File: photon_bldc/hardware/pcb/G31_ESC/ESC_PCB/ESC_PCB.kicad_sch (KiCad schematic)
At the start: 21 parts, among them J1 PWM_Input, J2 Motor_Plus, J3 Motor_Minus, J4 Conn_01x08, U1 STM32G431K6Ux, U2 AMS1117-5.0, U3 AMS1117-3.3, U4 74AHC1G86, U5 74AHC1G86

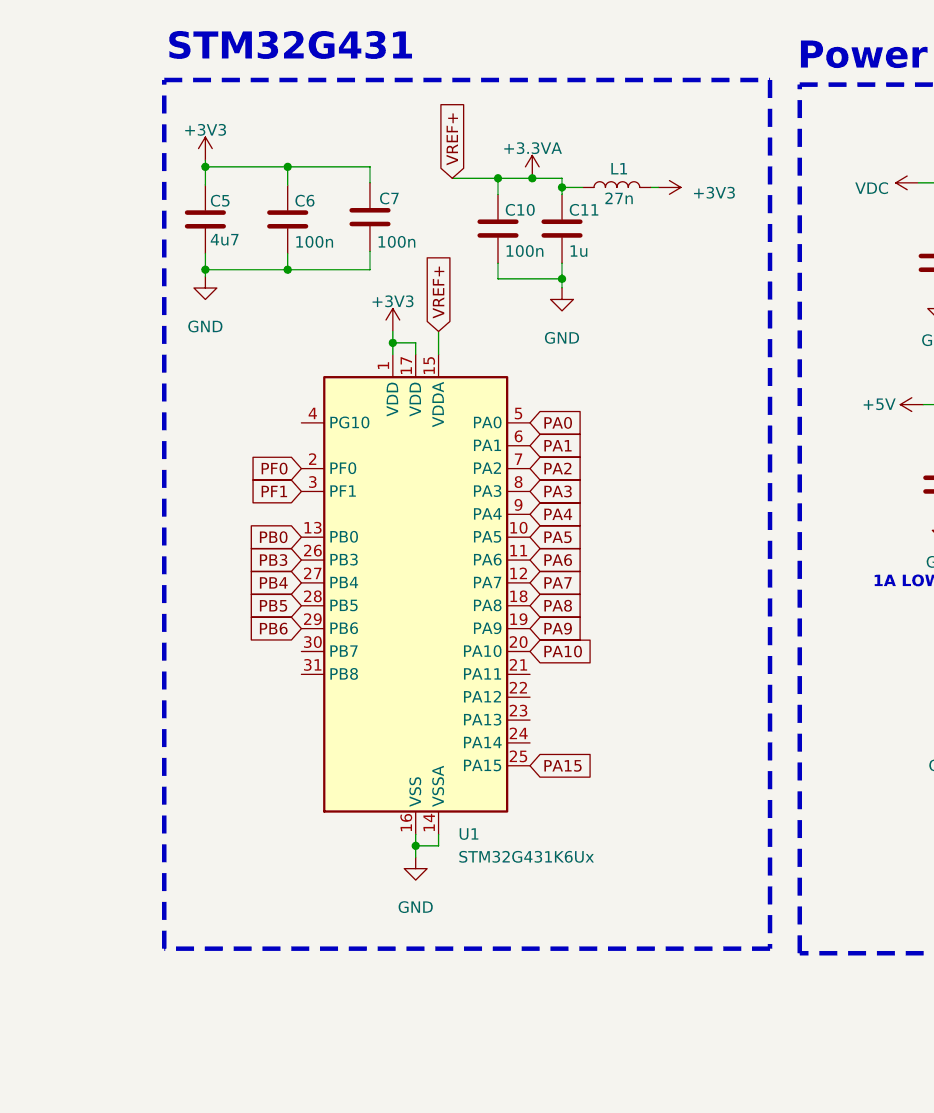
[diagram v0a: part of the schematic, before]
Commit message: g071
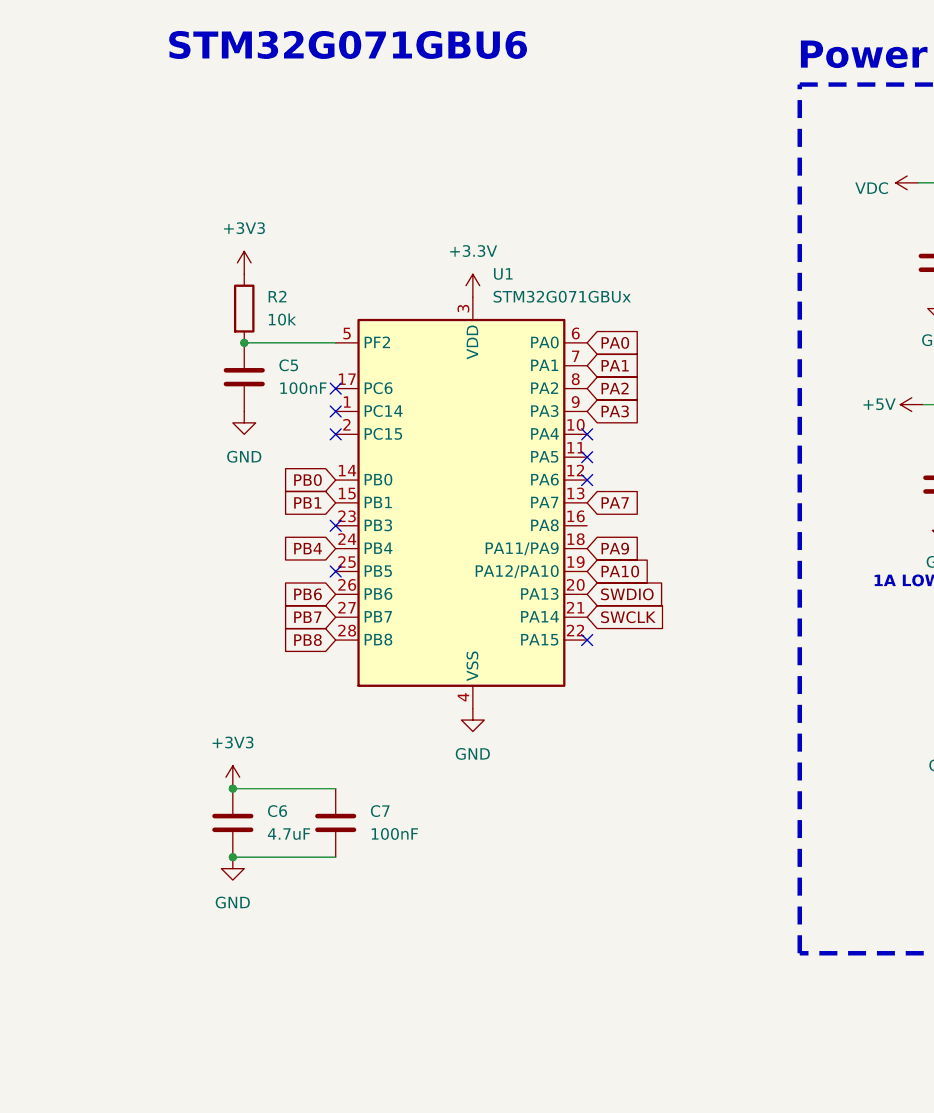
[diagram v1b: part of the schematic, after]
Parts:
- removed C10: 100n, Capacitor_SMD:C_0603_1608Metric, symbol Device:C
- removed C11: 1u, Capacitor_SMD:C_0603_1608Metric, symbol Device:C
- removed L1: 27n, Inductor_SMD:L_0603_1608Metric, symbol Device:L
- removed U1: STM32G431K6Ux, Package_DFN_QFN:QFN-32-1EP_5x5mm_P0.5mm_EP3.45x3.45mm, symbol MCU_ST_STM32G4:STM32G431K6Ux
- added R2: 10k, symbol Device:R
- added U1: STM32G071GBUx, Package_DFN_QFN:QFN-28_4x4mm_P0.5mm, symbol MCU_ST_STM32G0:STM32G071GBUx
- C5: value 4u7 -> 100nF; footprint Capacitor_SMD:C_0603_1608Metric -> (none)
- C6: value 100n -> 4.7uF; footprint Capacitor_SMD:C_0603_1608Metric -> (none)
- C7: value 100n -> 100nF; footprint Capacitor_SMD:C_0603_1608Metric -> (none)
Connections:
- net +3V3: now also R2.1; no longer C5.1
- net GND: now also U1.4 (VSS)
- net PA0: now also U1.6 (PA0)
- net PA1: now also U1.7 (PA1)
- net PA10: now also U1.19 (PA12/PA10)
- net PA2: now also U1.8 (PA2)
- net PA3: now also U1.9 (PA3)
- net PA7: now also U1.13 (PA7)
- net PA9: now also U1.18 (PA11/PA9)
- net PB0: now also U1.14 (PB0)
- net PB4: now also U1.24 (PB4)
- net PB6: now also U1.26 (PB6)
- new net: C5.1, R2.2, U1.5 (PF2)
- new net +3.3V: U1.3 (VDD)
- new net PB1: U1.15 (PB1)
- new net PB7: U1.27 (PB7)
- new net PB8: U1.28 (PB8)
- new net SWCLK: U1.21 (PA14)
- new net SWDIO: U1.20 (PA13)
- no-connect marks 0 -> 9
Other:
- note added: "STM32G071GBU6"
- note removed: "STM32G431"

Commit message: ESC schemat continued
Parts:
- added C10, C11, C9: 1uF, symbol Device:C
- added D1, D2, D3: D, symbol Device:D
- added Q1, Q2, Q3, Q4, Q5, Q6: NMOS, symbol Simulation_SPICE:NMOS
- added U6: ~, Fortior Tech FD6288Q driver library:QFN50P400X400X90-25N, symbol ESC library:FD6288Q
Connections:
- net GND: now also Q4.3 (S), Q5.3 (S), Q6.3 (S), U6.6 (COM)
- net VDC: now also Q1.1 (D), Q2.1 (D), Q3.1 (D)
- new net: C9.1, D1.1 (K), U6.20 (VB1)
- new net: C9.2, U6.18 (VS1)
- new net: C11.2, U6.12 (VS3)
- new net: C11.1, D3.1 (K), U6.14 (VB3)
- new net: C10.2, U6.15 (VS2)
- new net: C10.1, D2.1 (K), U6.17 (VB2)
- new net +8V: D1.2 (A), D2.2 (A), D3.2 (A), U6.4 (VCC)
- new net A: Q1.3 (S), Q4.1 (D)
- new net B: Q3.3 (S), Q5.1 (D)
- new net C: Q2.3 (S), Q6.1 (D)
- new net GHA: Q1.2 (G), U6.22 (HIN1)
- new net GHB: Q3.2 (G), U6.23 (HIN2)
- new net GHC: Q2.2 (G), U6.24 (HIN3)
- new net GLA: Q4.2 (G), U6.1 (LIN1)
- new net GLB: Q5.2 (G), U6.2 (LIN2)
- new net GLC: Q6.2 (G), U6.3 (LIN3)
- no-connect marks 9 -> 12
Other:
- moved on the sheet: C1, C2, C3, C4, C5, C6, C7, C8, J1, J2, J3, J4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

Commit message: 0.0
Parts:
- removed C8: C, symbol Device:C
- removed J1: PWM_Input, symbol Connector_Generic:Conn_01x02
- removed J4: Conn_01x08, symbol Connector_Generic:Conn_01x08
- removed R1: 10K, symbol Device:R
- removed U4, U5: 74AHC1G86, symbol 74xGxx:74AHC1G86
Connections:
- net +8V is gone; now on net +3V3: D1.2 (A), D2.2 (A), D3.2 (A), U6.4 (VCC)
- net PB7 is gone; now on net BEMF_REF: U1.27 (PB7)
- net GHA: now also U6.19 (HO1); no longer U6.22 (HIN1)
- net GHB: now also U6.16 (HO2); no longer U6.23 (HIN2)
- net GHC: now also U6.13 (HO3); no longer U6.24 (HIN3)
- net GLA: now also U6.11 (LO1); no longer U6.1 (LIN1)
- net GLB: now also U6.10 (LO2); no longer U6.2 (LIN2)
- net GLC: now also U6.9 (LO3); no longer U6.3 (LIN3)
- net HA: now reaches U1.16 (PA8)
- net HA: now also U6.22 (HIN1)
- net PA0 renamed BEMF_REF
- net PA1 renamed BEMF_A
- net PA10 renamed HC
- net HC: now also U6.24 (HIN3)
- net PA3 renamed BEMF_B
- net PA7: no longer names the net of U1.13 (PA7)
- net PA9 renamed HB
- net HB: now also U6.23 (HIN2)
- net PB0 renamed LB
- net LB: now also U6.2 (LIN2)
- net PB1 renamed LC
- net LC: now also U6.3 (LIN3)
- net PB4 renamed BEMF_C
- new net LA: U6.1 (LIN1)
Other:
- note added: "Mosfet Driver"
- moved on the sheet: C5, Q1, Q2, Q3, Q4, Q5, Q6, R2, U1
